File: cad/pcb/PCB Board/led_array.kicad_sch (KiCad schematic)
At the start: 20 parts

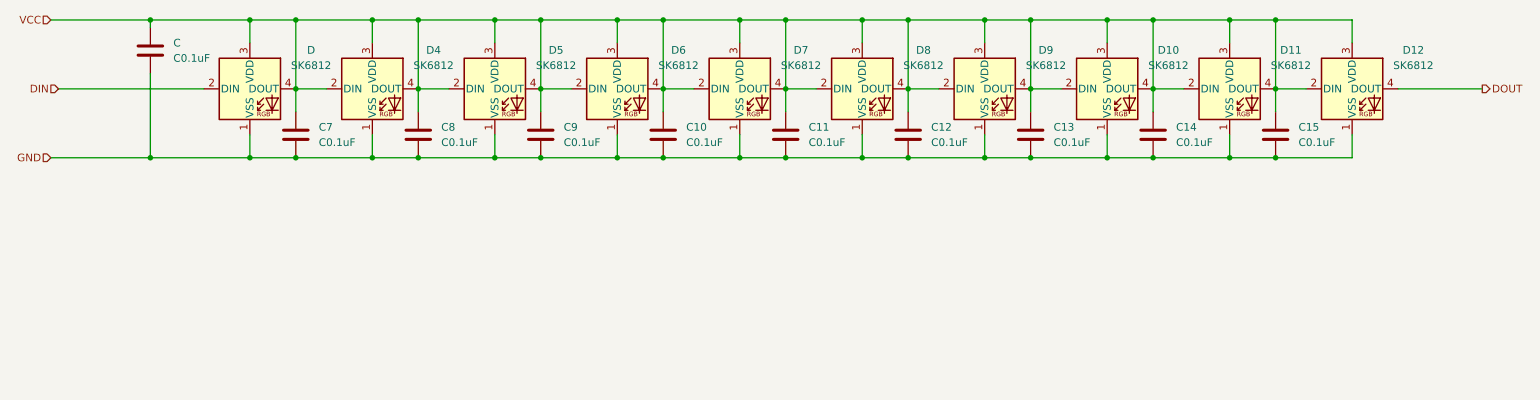
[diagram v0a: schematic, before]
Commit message: [WIP] save changes
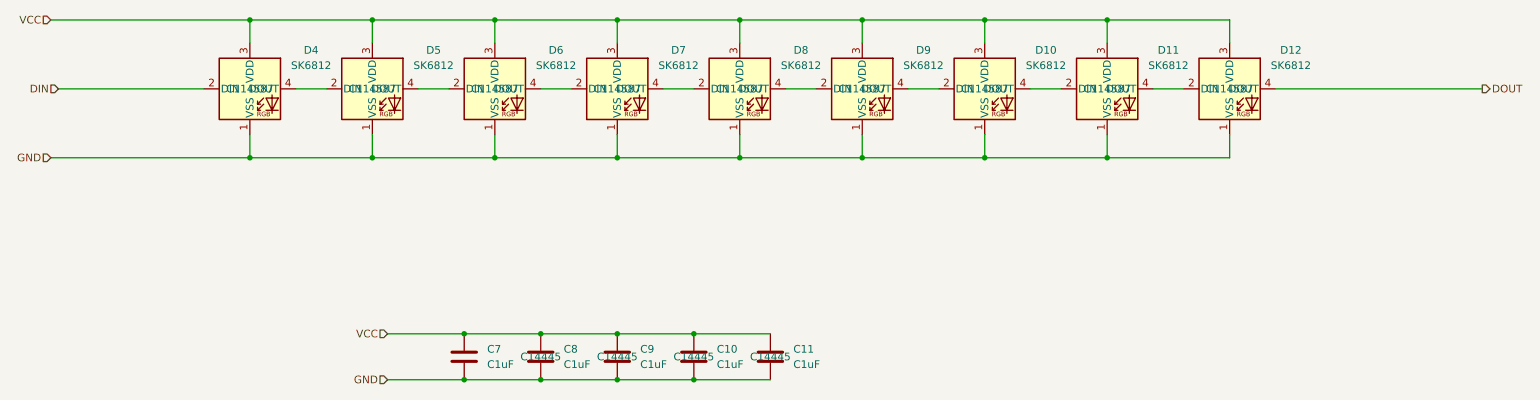
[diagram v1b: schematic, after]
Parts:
- removed C, C12, C13, C14, C15: C0.1uF, Capacitor_SMD:C_0402_1005Metric, symbol Device:C
- removed D12: SK6812, LED_SMD:LED_SK6812_PLCC4_5.0x5.0mm_P3.2mm, symbol LED:SK6812
- C10, C11, C7, C8, C9: value C0.1uF -> C1uF; LCSC (none) -> C14445
- D10: renamed from D9; LCSC (none) -> C114587
- D11: renamed from D10; LCSC (none) -> C114587
- D12: renamed from D11; LCSC (none) -> C114587
- D4: renamed from D; LCSC (none) -> C114587
- D5: renamed from D4; LCSC (none) -> C114587
- D6: renamed from D5; LCSC (none) -> C114587
- D7: renamed from D6; LCSC (none) -> C114587
- D8: renamed from D7; LCSC (none) -> C114587
- D9: renamed from D8; LCSC (none) -> C114587
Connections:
- net DOUT: now also D12.4 (DOUT)
- net VCC: no longer D10.2 (DIN), D10.4 (DOUT), D11.2 (DIN), D11.4 (DOUT), D12.2 (DIN), D12.4 (DOUT), D4.4 (DOUT), D5.2 (DIN), D5.4 (DOUT), D6.2 (DIN), D6.4 (DOUT), D7.2 (DIN), D7.4 (DOUT), D8.2 (DIN), D8.4 (DOUT), D9.2 (DIN), D9.4 (DOUT)
- new net: D4.4 (DOUT), D5.2 (DIN)
- new net: D5.4 (DOUT), D6.2 (DIN)
- new net: D8.4 (DOUT), D9.2 (DIN)
- new net: D10.2 (DIN), D9.4 (DOUT)
- new net: D11.4 (DOUT), D12.2 (DIN)
- new net: D6.4 (DOUT), D7.2 (DIN)
- new net: D7.4 (DOUT), D8.2 (DIN)
- new net: D10.4 (DOUT), D11.2 (DIN)
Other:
- moved on the sheet: C7
